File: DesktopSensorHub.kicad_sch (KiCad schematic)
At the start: 18 parts, among them J1 USB_C_Receptacle_USB2.0, SW1 SW_Push, U1 RP2040, U2 APDS-9960, U3 AP2112K-3.3, U4 W25Q16JVSS

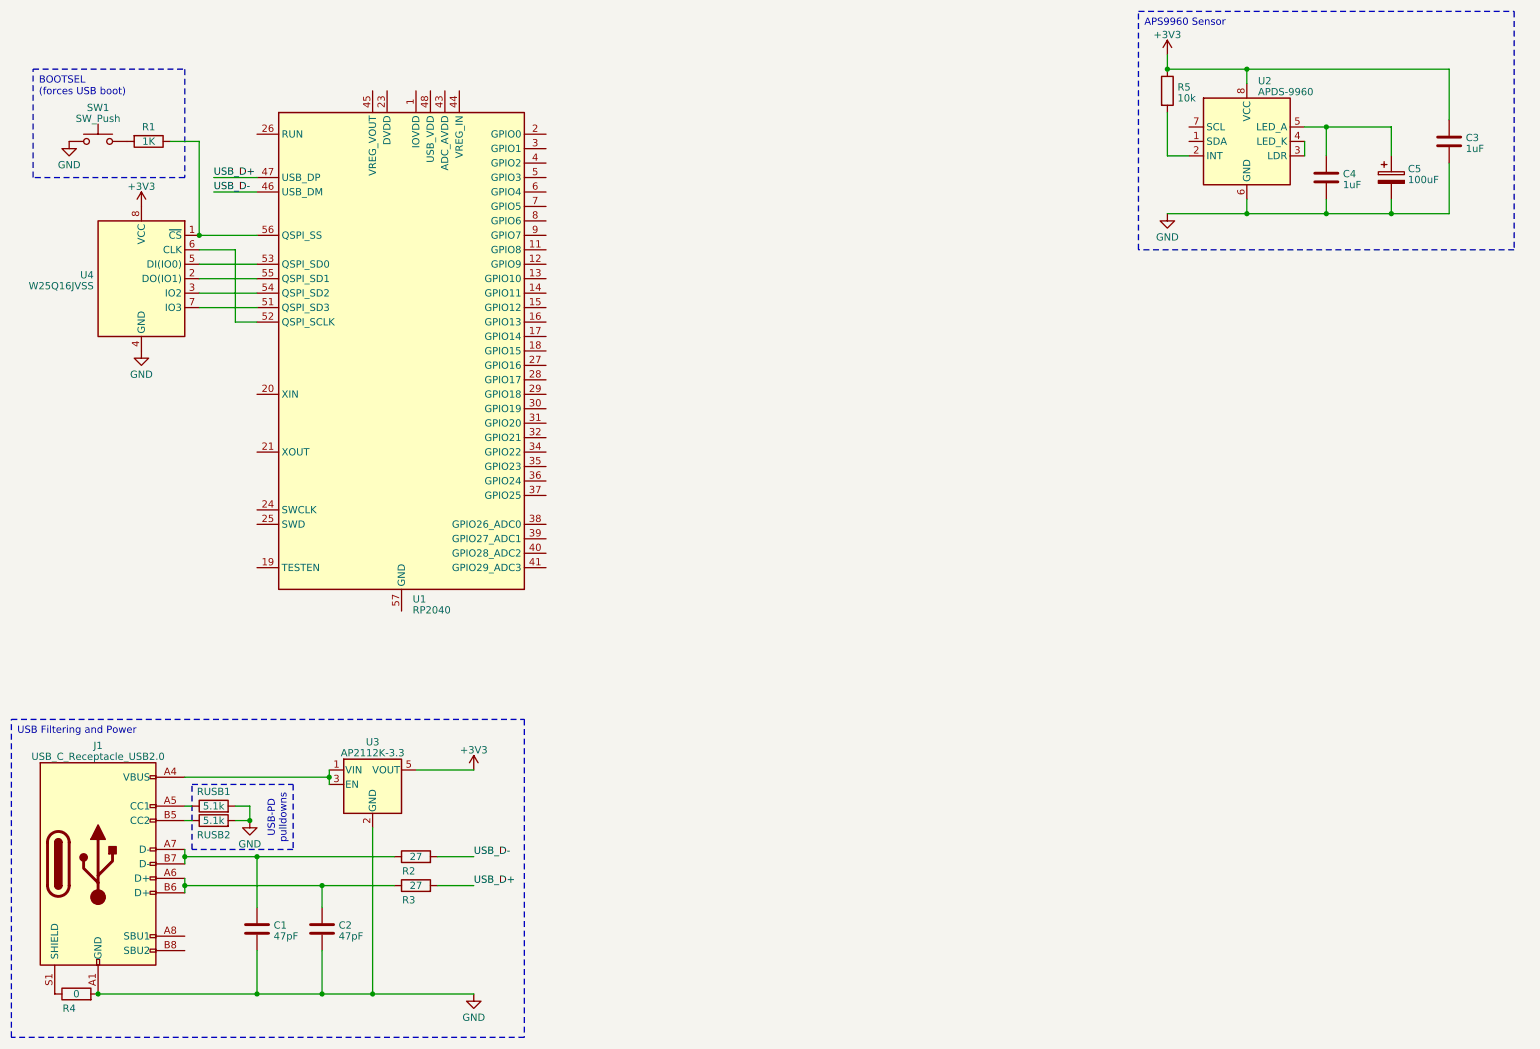
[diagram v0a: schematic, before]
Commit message: rev1 schematic finished
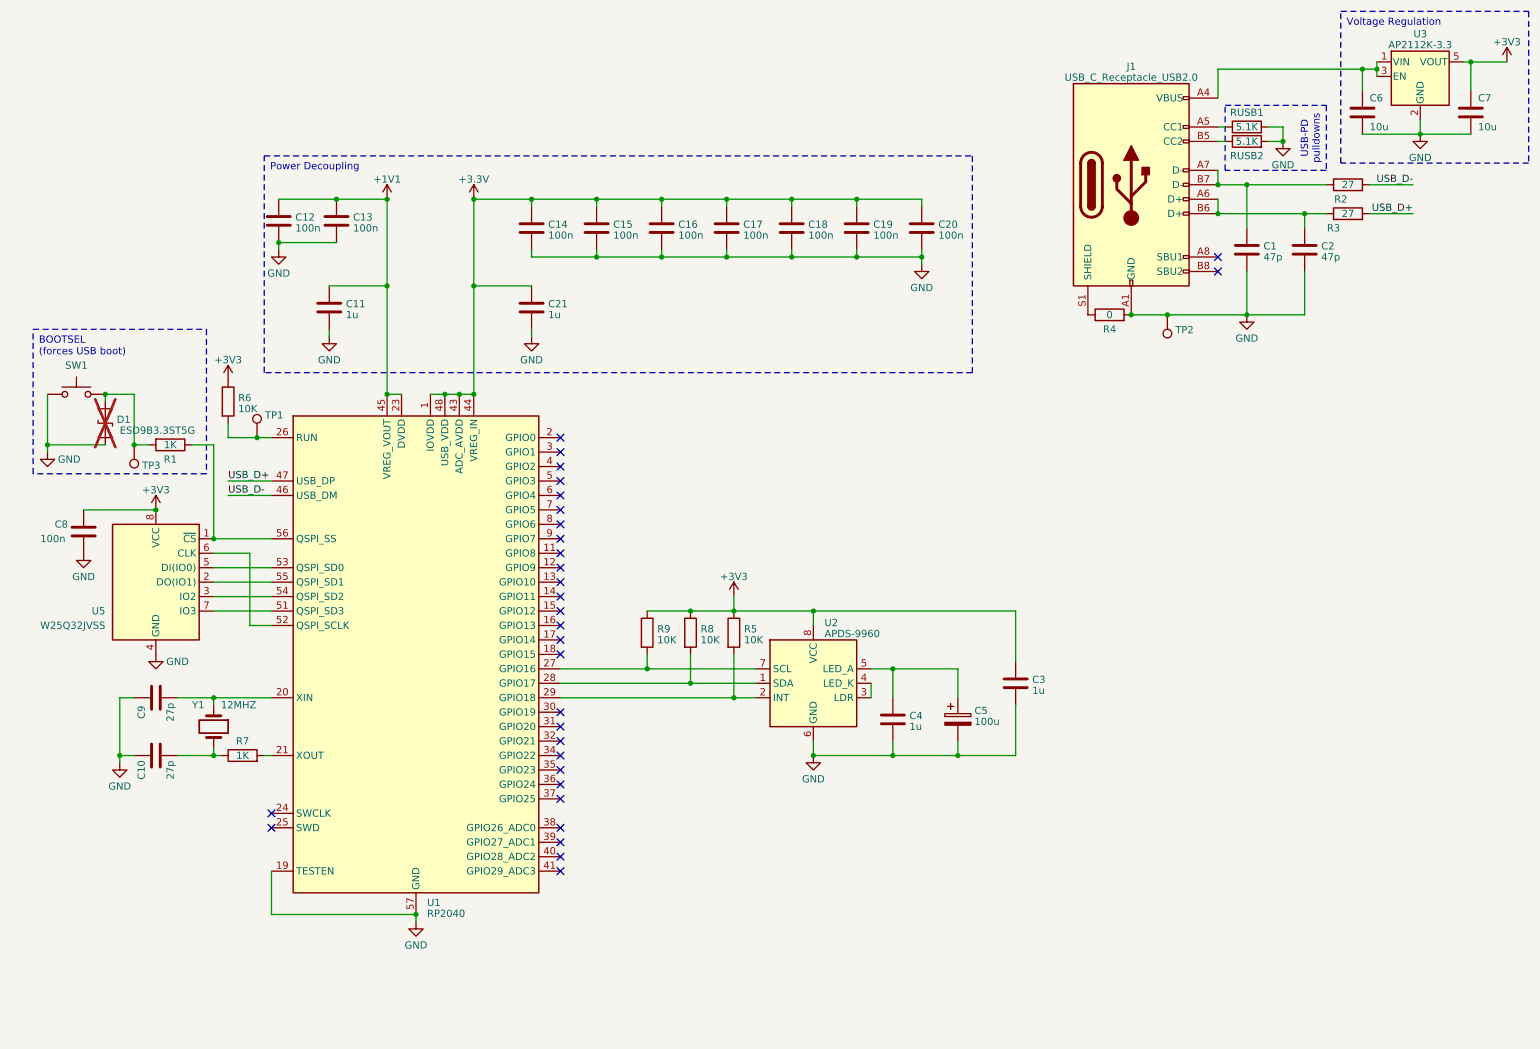
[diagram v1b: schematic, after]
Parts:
- removed U4: W25Q16JVSS, Package_SO:SOIC-8_5.23x5.23mm_P1.27mm, symbol W25Q16JVSS:W25Q16JVSS
- added C10, C9: 27p, symbol Device:C
- added C11, C21: 1u, symbol Device:C
- added C12, C13, C14, C15, C16, C17, C18, C19, C20, C8: 100n, symbol Device:C
- added C6, C7: 10u, symbol Device:C
- added D1: ESD9B3.3ST5G, Diode_SMD:D_SOD-923, symbol Diode:ESD9B3.3ST5G
- added R6, R8, R9: 10K, symbol Device:R
- added R7: 1K, symbol Device:R
- added TP1, TP2, TP3: TestPoint, symbol Connector:TestPoint
- added U5: W25Q32JVSS, Package_SO:SOIC-8_5.23x5.23mm_P1.27mm, symbol Memory_Flash:W25Q32JVSS
- added Y1: 12MHZ, Crystal:Crystal_SMD_HC49-SD, symbol Device:Crystal
- C1, C2: value 47pF -> 47p
- C3, C4: value 1uF -> 1u
- C5: value 100uF -> 100u
- R5: value 10k -> 10K
- RUSB1, RUSB2: value 5.1k -> 5.1K
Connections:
- net +3V3: now also C7.1, C8.1, R6.1, R8.1, R9.1, U5.8 (VCC)
- net GND: now also U1.19 (TESTEN), U1.57 (GND), C10.1, C11.2, C12.2, C13.2, C14.2, C15.2, C16.2, C17.2, C18.2, C19.2, C20.2, C21.2, C6.2, C7.2, C8.2, C9.1, D1.2 (A2), TP2.1, U5.4 (GND)
- net +3.3V: now reaches U1.1 (IOVDD), U1.10 (IOVDD), U1.22 (IOVDD), U1.33 (IOVDD), U1.42 (IOVDD), U1.49 (IOVDD)
- net +3.3V: now also U1.43 (ADC_AVDD), U1.44 (VREG_IN), U1.48 (USB_VDD), C14.1, C15.1, C16.1, C17.1, C18.1, C19.1, C20.1, C21.1
- net at U1.20 (XIN): now also C9.2, Y1.1
- net at U1.21 (XOUT): now also R7.2
- net +1V1: now reaches U1.23 (DVDD), U1.50 (DVDD)
- net +1V1: now also U1.45 (VREG_VOUT), C11.1, C12.1, C13.1
- net at U1.26 (RUN): now also R6.2, TP1.1
- net at U1.27 (GPIO16): now also U2.7 (SCL), R9.2
- net at U1.28 (GPIO17): now also U2.1 (SDA), R8.2
- net at U1.29 (GPIO18): now also R5.2, U2.2 (INT)
- net at U1.51 (QSPI_SD3): now also U5.7 (IO3)
- net at U1.52 (QSPI_SCLK): now also U5.6 (CLK)
- net at U1.53 (QSPI_SD0): now also U5.5 (DI(IO0))
- net at U1.54 (QSPI_SD2): now also U5.3 (IO2)
- net at U1.55 (QSPI_SD1): now also U5.2 (DO(IO1))
- net at R1.1, U1.56 (QSPI_SS): now also U5.1 (~{CS})
- net at J1.A4 (VBUS), J1.A9 (VBUS), J1.B4 (VBUS)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: now also C6.1
- net at R1.2, SW1.2: now also D1.1 (A1), TP3.1
- new net: C10.2, R7.1, Y1.2
- no-connect marks 0 -> 31
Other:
- moved on the sheet: C1, C2, C3, C4, C5, J1, R1, R2, R3, R4, R5, RUSB1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
